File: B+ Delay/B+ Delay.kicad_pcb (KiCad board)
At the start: 2 copper layers, 80 x 68 mm, 44 parts, among them J1 Pwr in, J2 B+ A, J3 B+ B, J4 LED, Q3 MMBT3904, Q4 MMBT3906, U1 LM7805_TO220, U2 SE556, U3 CPC1779, U4 CPC1779

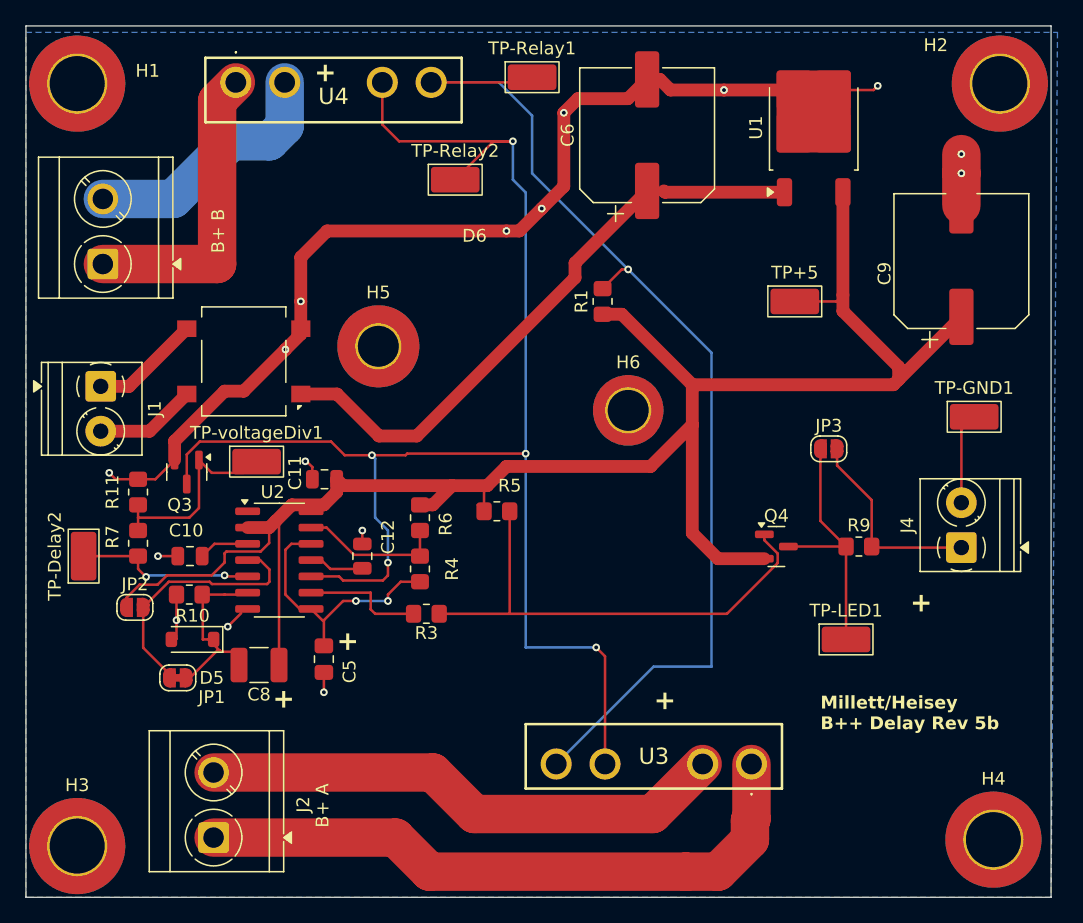
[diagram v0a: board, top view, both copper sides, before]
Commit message: Moving terminal block over
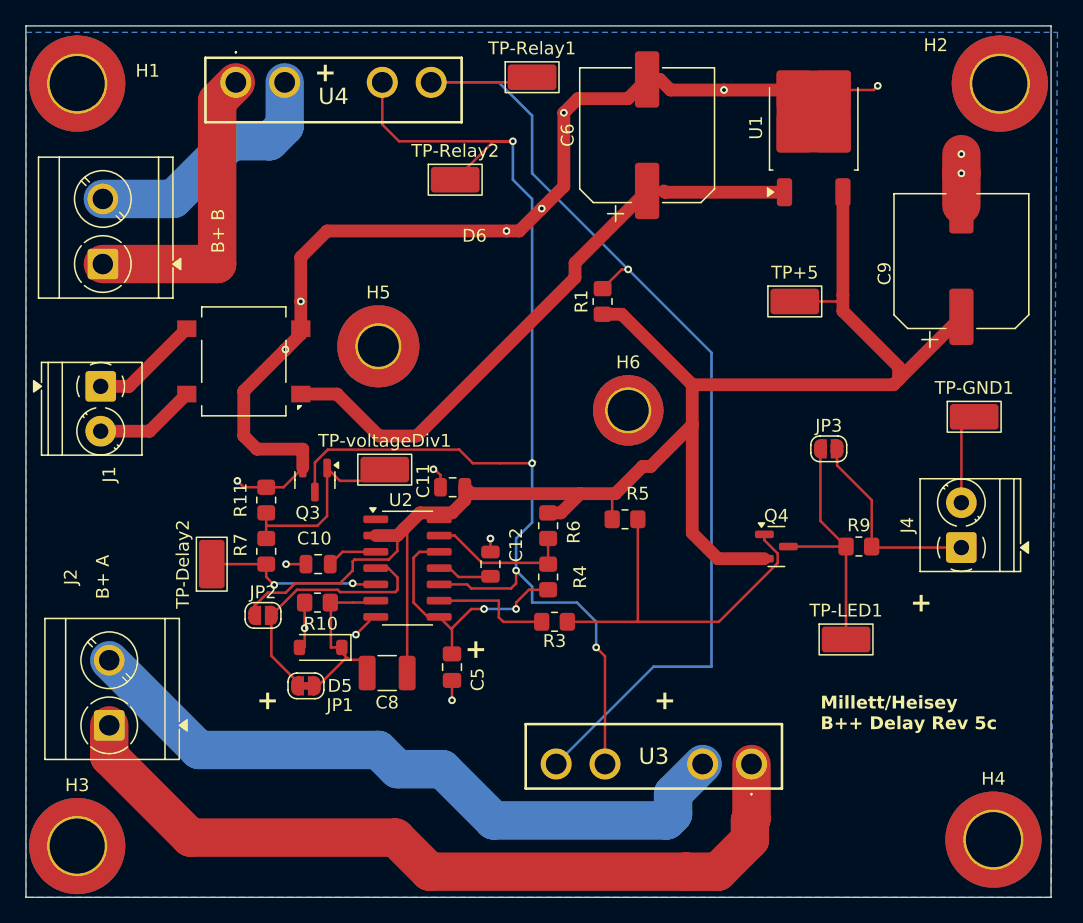
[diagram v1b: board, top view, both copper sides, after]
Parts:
- moved J2 12.0 mm to (156.5, -296.4)
- moved C10 10.0 mm to (172.8, -309.0)
- moved C11 10.0 mm to (183.3, -315.0)
- moved C12 10.0 mm to (186.2, -309.0)
- moved C5 10.0 mm to (183.2, -301.0)
- moved C8 10.0 mm to (178.2, -300.5)
- moved D5 10.0 mm to (173.0, -302.5)
- moved JP1 10.0 mm to (171.8, -299.5)
- moved JP2 10.0 mm to (168.5, -305.0)
- moved Q3 10.0 mm to (172.6, -315.6)
- moved R10 10.0 mm to (172.8, -306.0)
- moved R11 10.0 mm to (168.8, -314.0)
- moved R3 10.0 mm to (191.2, -304.5)
- moved R4 10.0 mm to (190.8, -308.0)
- moved R5 10.0 mm to (196.8, -312.5)
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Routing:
- net Net-(Q3-C): track 120.4 -> 102.1 mm, vias 5 -> 4
- net Net-(J2-Pin_1): track 49.9 -> 63.1 mm
- net A: track 41.1 -> 54.2 mm
- net +5V: track 143.1 -> 133.3 mm
- net Net-(Q4-B): track 38.7 -> 29.0 mm
- net GND: track 101.1 -> 102.6 mm
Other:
- board text added: "Millett/Heisey B++ Delay Rev 5c"
- board text removed: "Millett/Heisey B++ Delay Rev 5b"
